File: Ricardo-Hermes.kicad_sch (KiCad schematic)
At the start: 43 parts, among them J1 RBUS, U1 ESP32-S3, Y1 R940000171

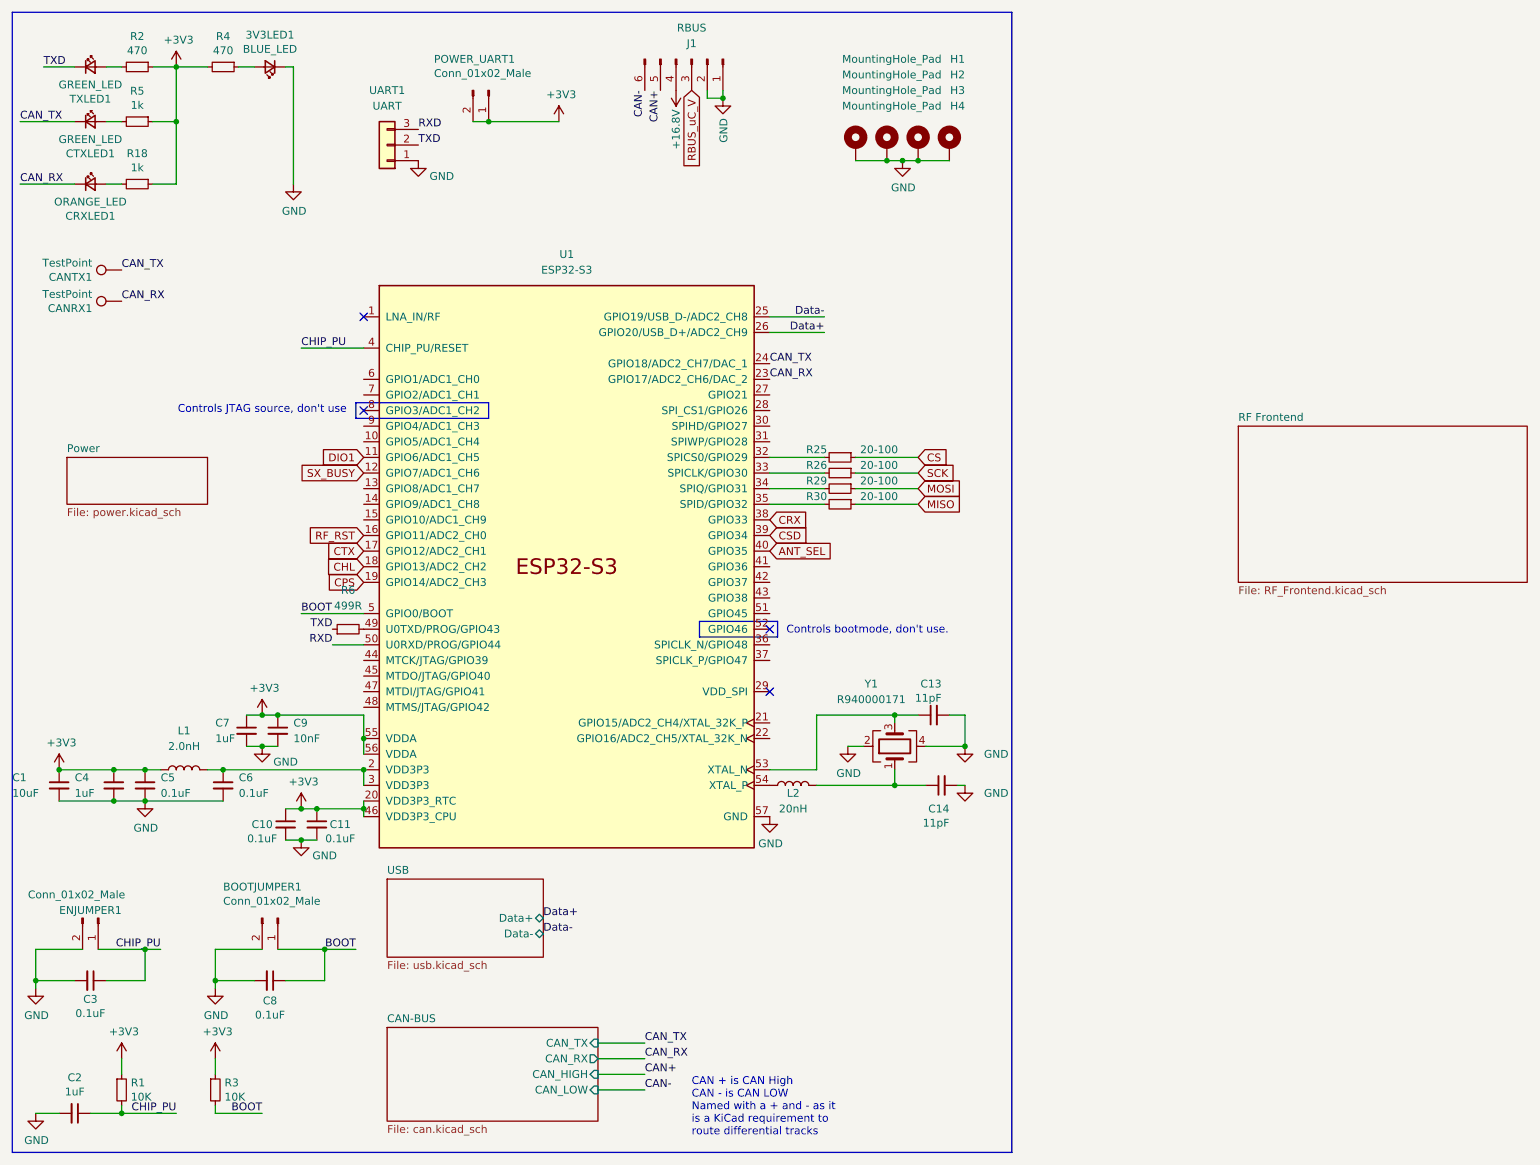
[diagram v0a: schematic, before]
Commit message: Post review changes WIP
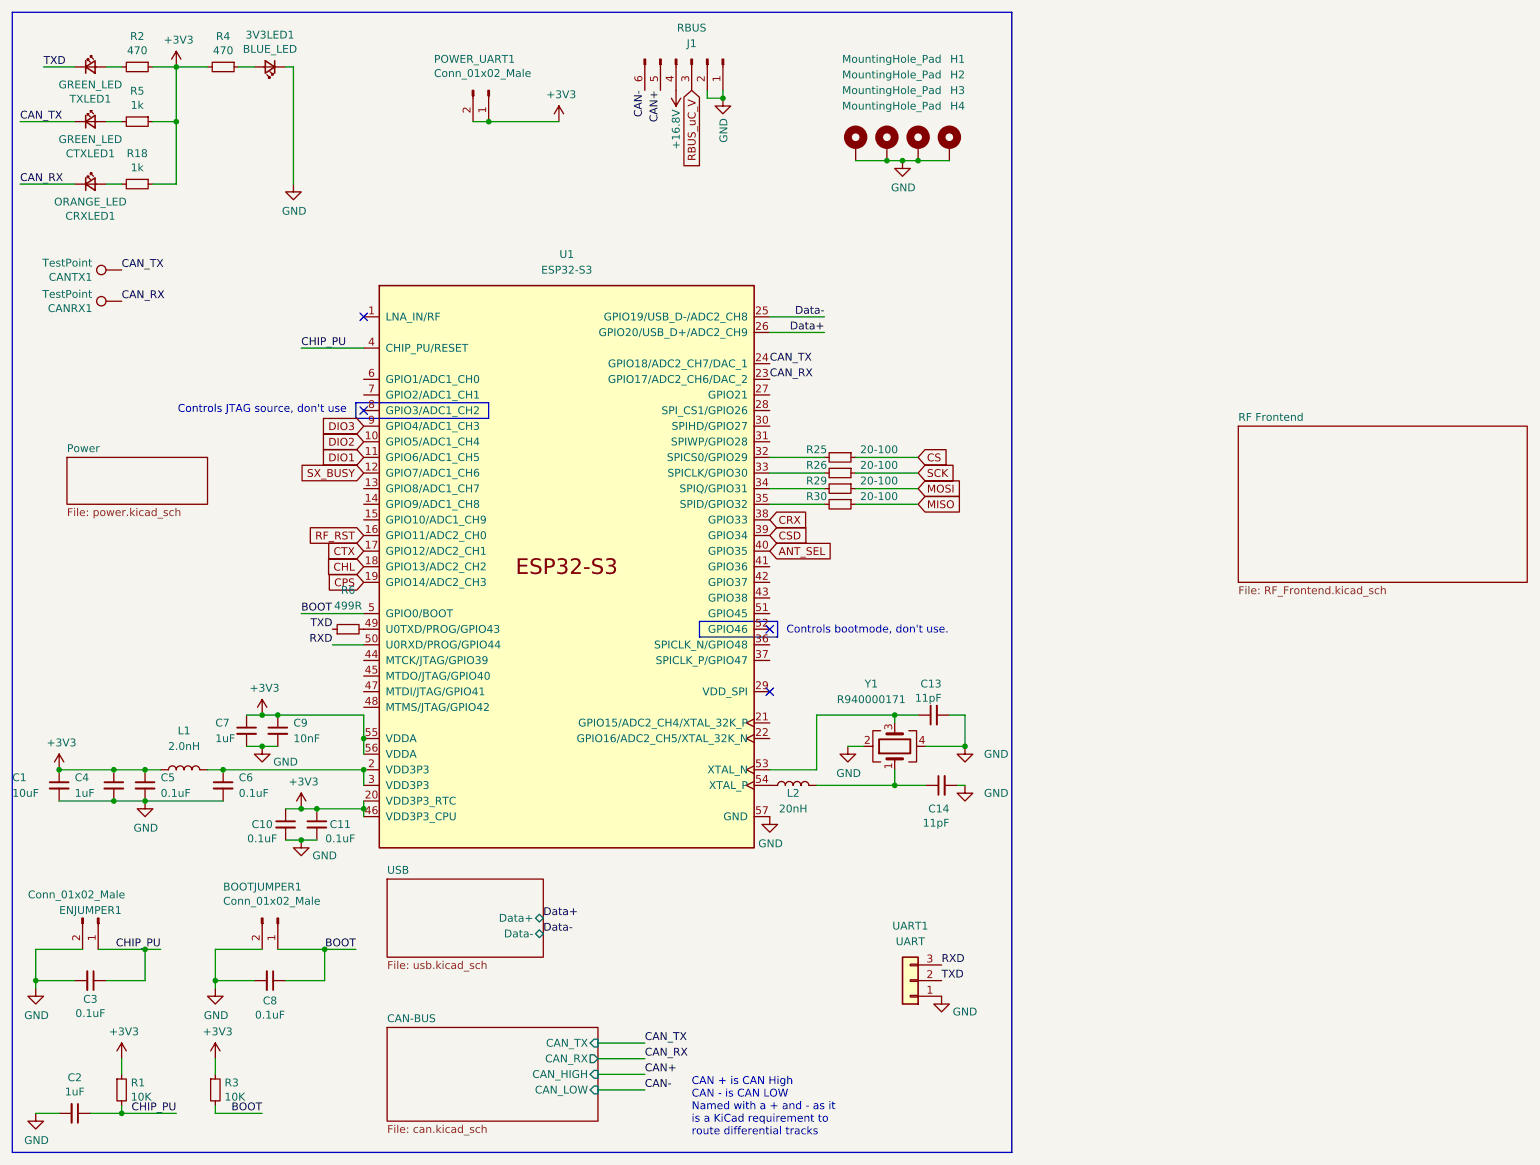
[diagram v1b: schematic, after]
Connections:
- net DIO2: now reaches U1.10 (GPIO5/ADC1_CH4)
- net DIO3: now reaches U1.9 (GPIO4/ADC1_CH3)
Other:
- moved on the sheet: UART1
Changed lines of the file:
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@@
 	)
 	(label "TXD"
-		(at 78.74 34.29 0)
+		(at 163.83 170.18 0)
 		(fields_autoplaced yes)
 		(effects
@@
 	)
 	(label "RXD"
-		(at 78.74 31.75 0)
+		(at 163.83 167.64 0)
 		(fields_autoplaced yes)
 		(effects
@@
 		)
 	)
+	(global_label "DIO3"
+		(shape input)
+		(at 69.85 80.01 180)
+		(fields_autoplaced yes)
+		(effects
+			(font
+				(size 1.27 1.27)
+			)
+			(justify right)
+		)
+		(property "Intersheetrefs" "${INTERSHEET_REFS}"
+			(at 63.1042 80.01 0)
+			(effects
+				(font
+					(size 1.27 1.27)
+				)
+				(justify right)
+				(hide yes)
+			)
+		)
+	)
+	(global_label "DIO2"
+		(shape input)
+		(at 69.85 82.55 180)
+		(fields_autoplaced yes)
+		(effects
+			(font
+				(size 1.27 1.27)
+			)
+			(justify right)
+		)
+		(property "Intersheetrefs" "${INTERSHEET_REFS}"
+			(at 63.1042 82.55 0)
+			(effects
+				(font
+					(size 1.27 1.27)
+				)
+				(justify right)
+				(hide yes)
+			)
+		)
+	)
 	(global_label "ANT_SEL"
 		(shape input)
@@
 	(symbol
 		(lib_id "power:GND")
-		(at 78.74 36.83 0)
+		(at 163.83 172.72 0)
 		(unit 1)
 		(exclude_from_sim no)
@@
 		(dnp no)
 		(property "Reference" "#PWR058"
-			(at 78.74 43.18 0)
+			(at 163.83 179.07 0)
 			(effects
 				(font
@@
 		)
 		(property "Value" "GND"
-			(at 82.55 39.37 0)
+			(at 167.64 175.26 0)
 			(effects
 				(font
@@
 		)
 		(property "Footprint" ""
-			(at 78.74 36.83 0)
+			(at 163.83 172.72 0)
 			(effects
 				(font
@@
 		)
 		(property "Datasheet" ""
-			(at 78.74 36.83 0)
+			(at 163.83 172.72 0)
 			(effects
 				(font
@@
 		)
 		(property "Description" ""
-			(at 78.74 36.83 0)
+			(at 163.83 172.72 0)
 			(effects
 				(font
@@
 	(symbol
 		(lib_id "Connector_Generic:Conn_01x03")
-		(at 73.66 34.29 180)
+		(at 158.75 170.18 180)
 		(unit 1)
 		(exclude_from_sim no)
@@
 		(fields_autoplaced yes)
 		(property "Reference" "UART1"
-			(at 73.66 25.4 0)
+			(at 158.75 161.29 0)
 			(effects
 				(font
@@
 		)
 		(property "Value" "UART"
-			(at 73.66 27.94 0)
+			(at 158.75 163.83 0)
 			(effects
 				(font
@@
 		)
 		(property "Footprint" "Connector_Molex:Molex_Nano-Fit_105313-xx03_1x03_P2.50mm_Horizontal"
-			(at 73.66 34.29 0)
+			(at 158.75 170.18 0)
 			(effects
 				(font
@@
 		)
 		(property "Datasheet" "~"
-			(at 73.66 34.29 0)
+			(at 158.75 170.18 0)
 			(effects
 				(font
@@
 		)
 		(property "Description" "Generic connector, single row, 01x03, script generated (kicad-library-utils/schlib/autogen/connector/)"
-			(at 73.66 34.29 0)
+			(at 158.75 170.18 0)
 			(effects
 				(font

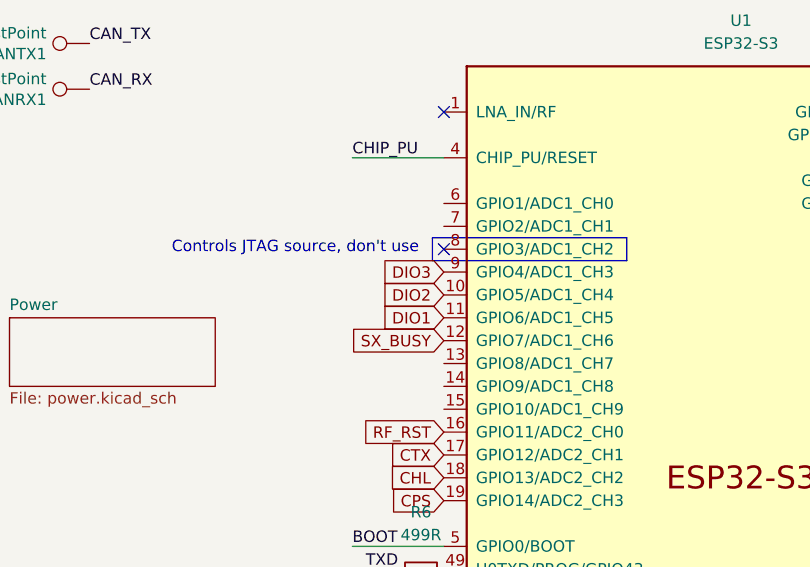
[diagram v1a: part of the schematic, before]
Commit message: Minor fixes
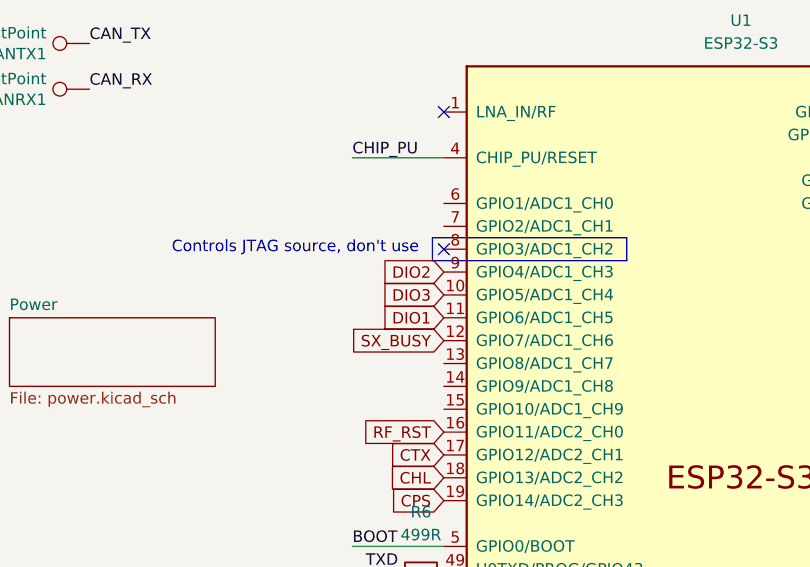
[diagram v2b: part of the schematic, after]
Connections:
- net DIO2: now also U1.9 (GPIO4/ADC1_CH3); no longer U1.10 (GPIO5/ADC1_CH4)
- net DIO3: now also U1.10 (GPIO5/ADC1_CH4); no longer U1.9 (GPIO4/ADC1_CH3)
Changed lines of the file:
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@@
 	(global_label "DIO3"
+		(shape input)
+		(at 69.85 82.55 180)
+		(fields_autoplaced yes)
+		(effects
+			(font
+				(size 1.27 1.27)
+			)
+			(justify right)
+		)
+		(property "Intersheetrefs" "${INTERSHEET_REFS}"
+			(at 63.1042 82.55 0)
+			(effects
+				(font
+					(size 1.27 1.27)
+				)
+				(justify right)
+				(hide yes)
+			)
+		)
+	)
+	(global_label "DIO2"
 		(shape input)
 		(at 69.85 80.01 180)
@@
 			(effects
 				(font
-					(size 1.27 1.27)
-				)
-				(justify right)
-				(hide yes)
-			)
-		)
-	)
-	(global_label "DIO2"
-		(shape input)
-		(at 69.85 82.55 180)
-		(fields_autoplaced yes)
-		(effects
-			(font
-				(size 1.27 1.27)
-			)
-			(justify right)
-		)
-		(property "Intersheetrefs" "${INTERSHEET_REFS}"
-			(at 63.1042 82.55 0)
-			(effects
-				(font
